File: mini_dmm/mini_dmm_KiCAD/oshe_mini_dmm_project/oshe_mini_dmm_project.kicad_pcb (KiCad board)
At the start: 2 copper layers, 2 parts, among them U1 LM324, U2 STM32F303CBTx

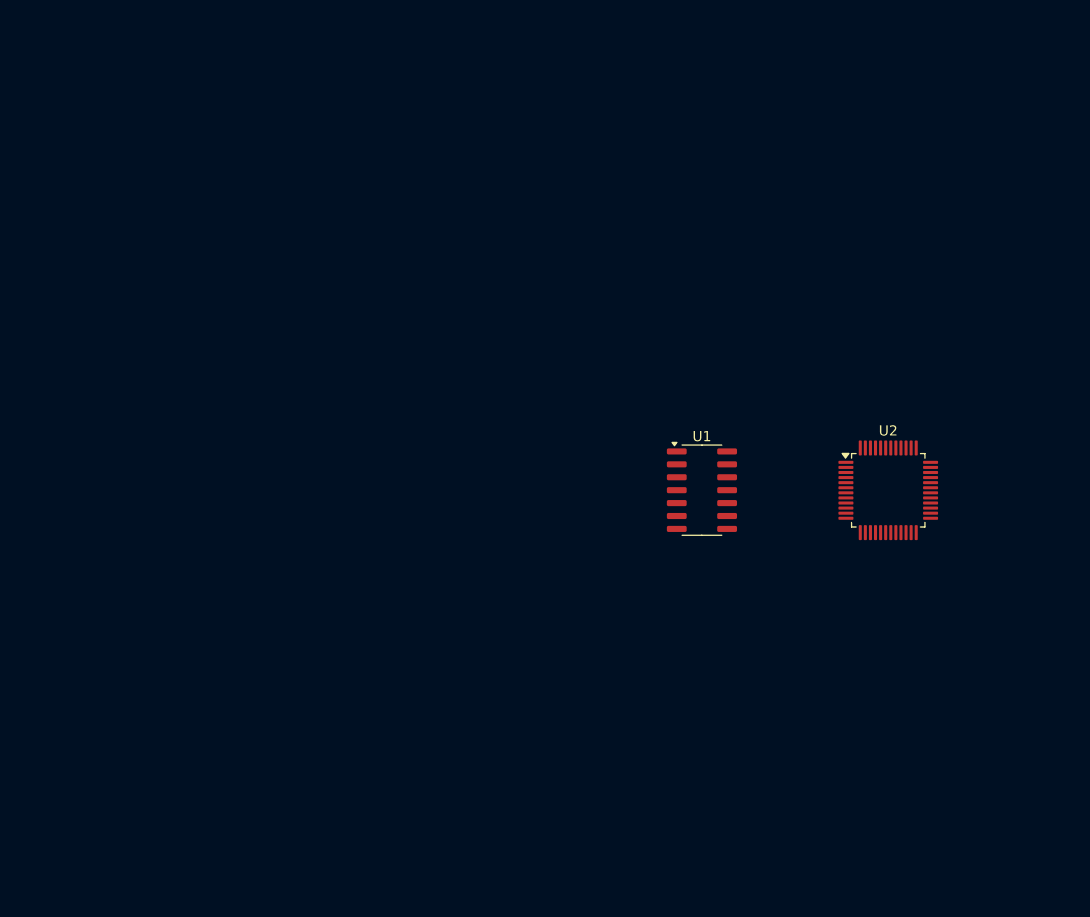
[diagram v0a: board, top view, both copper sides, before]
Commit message: Made some more changes
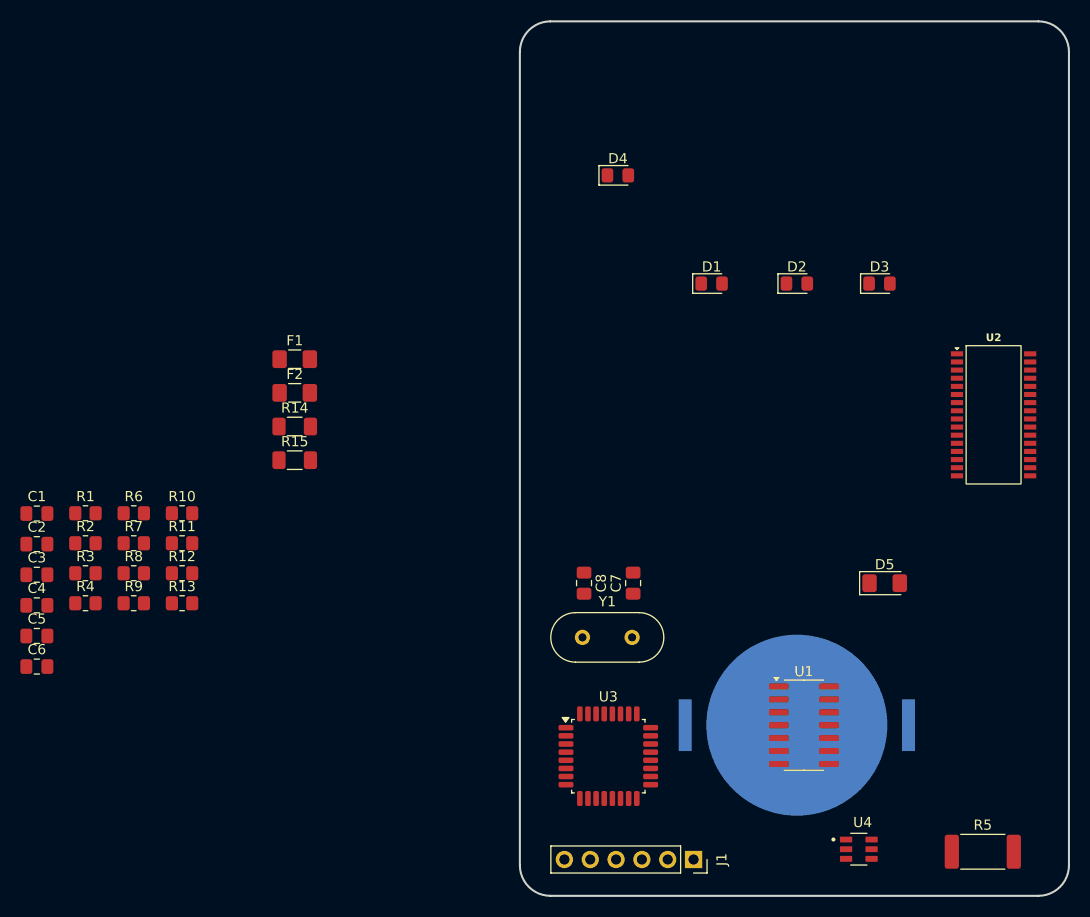
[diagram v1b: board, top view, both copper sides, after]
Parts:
- added BT1: Battery, Battery:BatteryHolder_Keystone_3034_1x20mm, B.Cu at (145.8, 119.4)
- added C1: 0.1uF, Capacitor_SMD:C_0805_2012Metric_Pad1.18x1.45mm_HandSolder, F.Cu at (71.1, 98.6)
- added C2: 1uF, Capacitor_SMD:C_0805_2012Metric_Pad1.18x1.45mm_HandSolder, F.Cu at (71.1, 101.6)
- added C3: 0.1uF, Capacitor_SMD:C_0805_2012Metric_Pad1.18x1.45mm_HandSolder, F.Cu at (71.1, 104.6)
- added C4: 1uF, Capacitor_SMD:C_0805_2012Metric_Pad1.18x1.45mm_HandSolder, F.Cu at (71.1, 107.6)
- added C5: 1uF, Capacitor_SMD:C_0805_2012Metric_Pad1.18x1.45mm_HandSolder, F.Cu at (71.1, 110.6)
- added C6: 0.1uF, Capacitor_SMD:C_0805_2012Metric_Pad1.18x1.45mm_HandSolder, F.Cu at (71.1, 113.6)
- added C7: 22pF, Capacitor_SMD:C_0805_2012Metric_Pad1.18x1.45mm_HandSolder, F.Cu at (129.7, 105.4)
- added C8: 22pF, Capacitor_SMD:C_0805_2012Metric_Pad1.18x1.45mm_HandSolder, F.Cu at (124.9, 105.4)
- added D1: VOLTAGE, LED_SMD:LED_0805_2012Metric_Pad1.15x1.40mm_HandSolder, F.Cu at (137.4, 75.9)
- added D2: CURRENT, LED_SMD:LED_0805_2012Metric_Pad1.15x1.40mm_HandSolder, F.Cu at (145.8, 75.9)
- added D3: RESISTANCE, LED_SMD:LED_0805_2012Metric_Pad1.15x1.40mm_HandSolder, F.Cu at (153.9, 75.9)
- added D4: NEGATIVE, LED_SMD:LED_0805_2012Metric_Pad1.15x1.40mm_HandSolder, F.Cu at (128.2, 65.3)
- added D5: Green, LED_SMD:LED_1206_3216Metric_Pad1.42x1.75mm_HandSolder, F.Cu at (154.4, 105.4)
- added F1: 500mA, Fuse:Fuse_1206_3216Metric_Pad1.42x1.75mm_HandSolder, F.Cu at (96.4, 83.4)
- added F2: 1A, Fuse:Fuse_1206_3216Metric_Pad1.42x1.75mm_HandSolder, F.Cu at (96.4, 86.7)
- added J1: FTDI Basic, Connector_PinSocket_2.54mm:PinSocket_1x06_P2.54mm_Vertical, F.Cu at (135.6, 132.6)
- added R1: 9.1MEG, Resistor_SMD:R_0805_2012Metric_Pad1.20x1.40mm_HandSolder, F.Cu at (75.8, 98.5)
- added R10: 1k, Resistor_SMD:R_0805_2012Metric_Pad1.20x1.40mm_HandSolder, F.Cu at (85.3, 98.5)
- added R11: 1k, Resistor_SMD:R_0805_2012Metric_Pad1.20x1.40mm_HandSolder, F.Cu at (85.3, 101.5)
- added R12: 1k, Resistor_SMD:R_0805_2012Metric_Pad1.20x1.40mm_HandSolder, F.Cu at (85.3, 104.4)
- added R13: 1k, Resistor_SMD:R_0805_2012Metric_Pad1.20x1.40mm_HandSolder, F.Cu at (85.3, 107.4)
- added R14: 390, Resistor_SMD:R_1206_3216Metric_Pad1.30x1.75mm_HandSolder, F.Cu at (96.4, 90.0)
- added R15: 10k, Resistor_SMD:R_1206_3216Metric_Pad1.30x1.75mm_HandSolder, F.Cu at (96.4, 93.3)
- added R2: 1MEG, Resistor_SMD:R_0805_2012Metric_Pad1.20x1.40mm_HandSolder, F.Cu at (75.8, 101.5)
- added R3: 9.1MEG, Resistor_SMD:R_0805_2012Metric_Pad1.20x1.40mm_HandSolder, F.Cu at (75.8, 104.4)
- added R4: 1MEG, Resistor_SMD:R_0805_2012Metric_Pad1.20x1.40mm_HandSolder, F.Cu at (75.8, 107.4)
- added R5: 1, Resistor_SMD:R_2512_6332Metric_Pad1.40x3.35mm_HandSolder, F.Cu at (164.1, 131.8)
- added R6: 9.1MEG, Resistor_SMD:R_0805_2012Metric_Pad1.20x1.40mm_HandSolder, F.Cu at (80.6, 98.5)
- added R7: 1MEG, Resistor_SMD:R_0805_2012Metric_Pad1.20x1.40mm_HandSolder, F.Cu at (80.6, 101.5)
- added R8: 9.1MEG, Resistor_SMD:R_0805_2012Metric_Pad1.20x1.40mm_HandSolder, F.Cu at (80.6, 104.4)
- added R9: 1MEG, Resistor_SMD:R_0805_2012Metric_Pad1.20x1.40mm_HandSolder, F.Cu at (80.6, 107.4)
- added U3: ATmega328P-A, Package_QFP:TQFP-32_7x7mm_P0.8mm, F.Cu at (127.3, 122.4)
- added U4: LM2664M6, Mini_DMM_Footprint_Library:SOT95P280X145-6N, F.Cu at (151.9, 131.6)
- added Y1: 16MHz, Crystal:Crystal_HC49-U_Vertical, F.Cu at (124.7, 110.7)
- U2: value STM32F303CBTx -> BU91796FS-ME2; footprint Package_QFP:LQFP-48_7x7mm_P0.5mm -> Mini_DMM_Footprint_Library:SSOP-A32
- moved U1 25.2 mm to (146.5, 119.4)
- moved U2 12.7 mm to (165.1, 88.9)
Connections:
- net Node_1 renamed A0
- net Node_2 renamed A1
- net Node_3 renamed A2
- net Node_4 renamed A3
- U2 pad 23: Net-(U2-VSS-Pad23) -> unconnected-(U2-VLCD-Pad23)
- U2 pad 24: unconnected-(U2-VDD-Pad24) -> +3.3V
- U2 pad 25: unconnected-(U2-PB12-Pad25) -> GND
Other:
- board outline added: 54 x 86 mm
